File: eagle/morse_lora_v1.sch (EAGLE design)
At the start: 20 parts

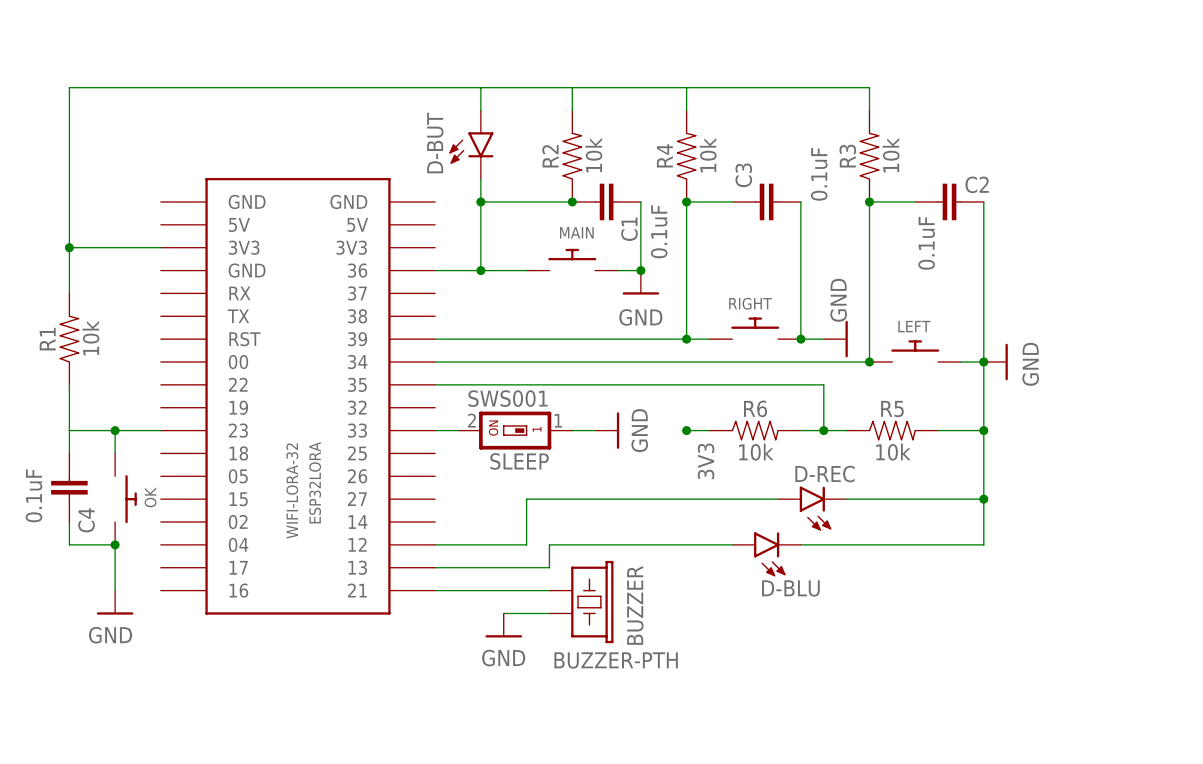
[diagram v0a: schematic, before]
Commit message: draft layout
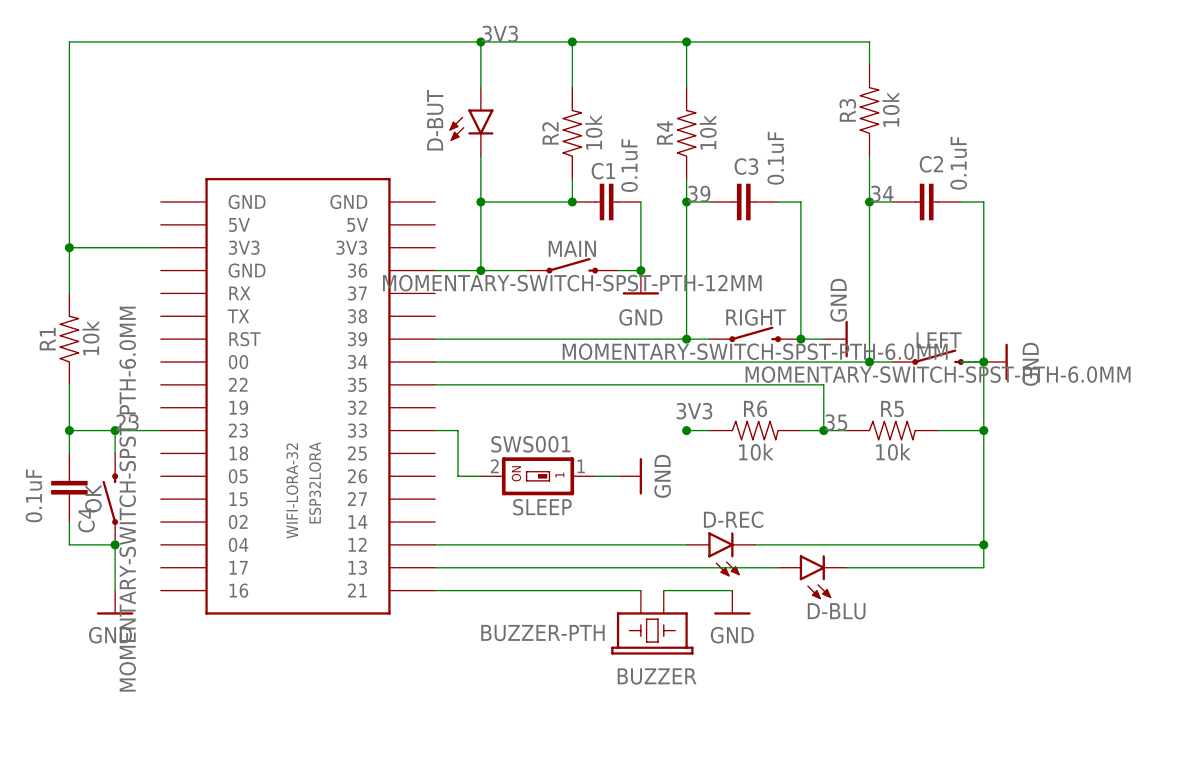
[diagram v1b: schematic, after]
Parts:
- LEFT, OK, RIGHT: value (none) -> MOMENTARY-SWITCH-SPST-PTH-6.0MM; device adafruit:SWITCH_PUSHBUTTONEVQ-PE -> SparkFun-Switches:MOMENTARY-SWITCH-SPST-PTH-6.0MM
- MAIN: value (none) -> MOMENTARY-SWITCH-SPST-PTH-12MM; device adafruit:SWITCH_PUSHBUTTONEVQ-PE -> SparkFun-Switches:MOMENTARY-SWITCH-SPST-PTH-12MM
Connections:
- net N$12 renamed 35
- removed net 3V3@1: ESP32LORA.3V3@1, R1.2, R3.2
- removed net N$1: C1.2, D-BUT.C, R2.1
- removed net N$10: R2.2
- removed net N$11: R4.2
- removed net N$2: C3.1, ESP32LORA.39, R4.1, RIGHT.P$1
- removed net N$3: C2.2, ESP32LORA.34, LEFT.P$1, R3.1
- removed net N$7: C4.2, ESP32LORA.23, OK.P$1, R1.1
- removed net N$8: ESP32LORA.36, MAIN.P$1
- removed net N$9: D-BUT.A
- new net 23: C4.2, ESP32LORA.23, OK.2, R1.1
- new net 34: C2.2, ESP32LORA.34, LEFT.1, R3.1
- new net 36: C1.2, D-BUT.C, ESP32LORA.36, MAIN.1, R2.1
- new net 39: C3.1, ESP32LORA.39, R4.1, RIGHT.1
- net 3V3: now also D-BUT.A, ESP32LORA.3V3@1, R1.2, R2.2, R3.2, R4.2
- net GND: now also LEFT.2, MAIN.2, OK.1, RIGHT.2; no longer LEFT.P$2, MAIN.P$2, OK.P$2, RIGHT.P$2
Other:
- moved on the sheet: BUZZER, C2, C3, D-BLU, D-BUT, D-REC, R2, R3, R4, SLEEP
